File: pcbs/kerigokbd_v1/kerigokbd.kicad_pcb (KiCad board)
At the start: 2 copper layers, 139.5 x 92 mm, 83 parts, among them J1 USB4520-03-0-A, J2 Conn_01x04, J3 Conn_01x03, J4 SJ-3501-SMT-TR, SW1 SW_Push, SW10 SW_Push, SW11 SW_Push, SW12 SW_Push, SW13 SW_Push, SW14 SW_Push, SW15 SW_Push, SW16 SW_Push, SW17 SW_Push, SW18 SW_Push, SW19 SW_Push, SW2 SW_Push, SW20 SW_Push, SW21 SW_Push, SW22 SW_Push, SW23 SW_Push, SW24 SW_Push, SW3 SW_Push, SW4 SW_Push, SW5 SW_Push, SW6 SW_Push, SW7 SW_Push, SW8 SW_Push, SW9 SW_Push, U1 TLV75533PDBVR, U2 RP2040, U3 W25Q16JVUXIQ, Y1 12MHz

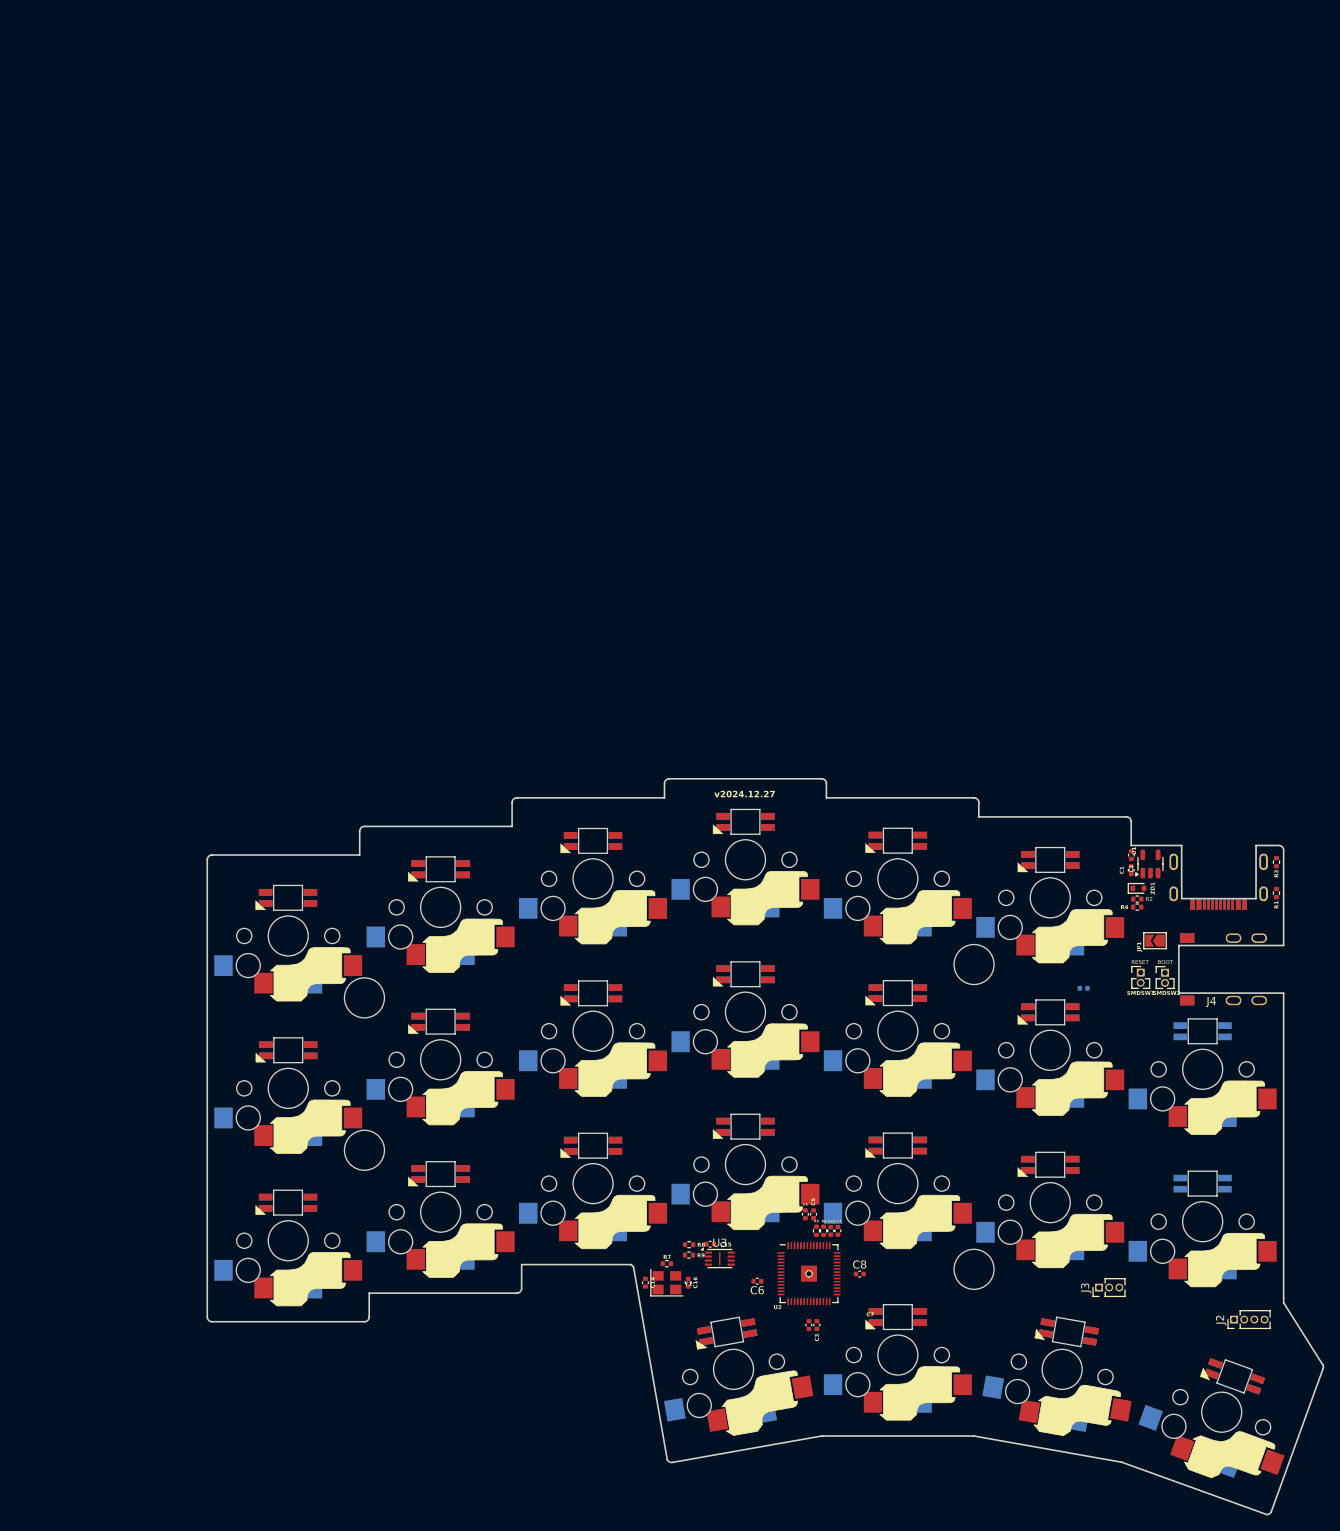
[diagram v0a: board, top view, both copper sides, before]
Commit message: update pcb
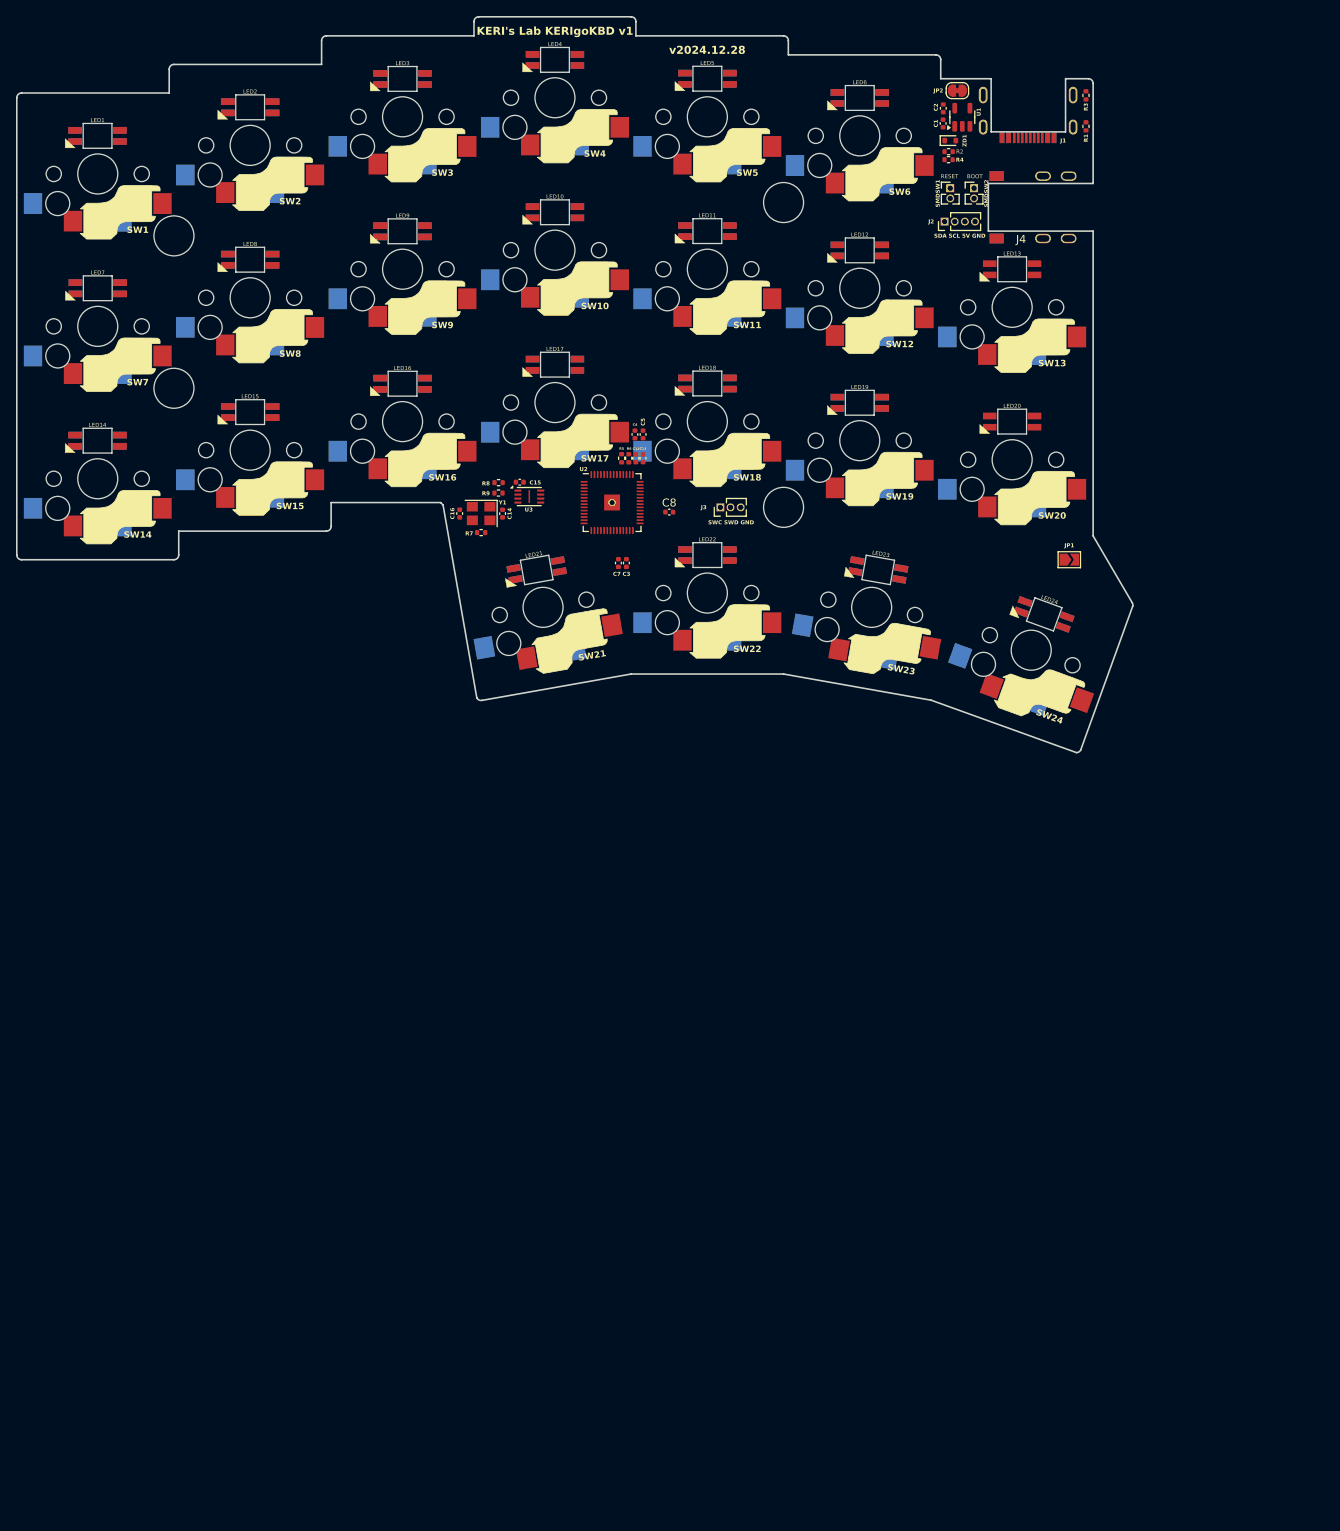
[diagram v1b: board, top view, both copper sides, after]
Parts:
- removed C11, C6: 100n, Capacitor_SMD:C_0402_1005Metric
- added JP2: LED_EN, Jumper:SolderJumper-2_P1.3mm_Bridged_RoundedPad1.0x1.5mm, F.Cu at (133.3, 24.4)
- J1, LED1, LED10, LED11, LED12, LED13, LED14, LED15, LED16, LED17, LED18, LED19, LED2, LED20, LED21, LED22, LED23, LED24, LED3, LED4, LED5, LED6, LED7, LED8, LED9, SW1, SW10, SW11, SW12, SW13, SW14, SW15, SW16, SW17, SW18, SW19, SW2, SW20, SW21, SW22, SW23, SW24, SW3, SW4, SW5, SW6, SW7, SW8, SW9: moved to F.Cu
- J2: value Conn_01x04 -> SDA SCL 5V GND
- J3: value Conn_01x03 -> SWC SWD GND
- moved J2 141.9 mm to (131.7, 40.7)
- moved J3 108.4 mm to (103.7, 76.5)
- moved SMDSW2 100.9 mm to (135.4, 36.6)
- moved SMDSW1 100.9 mm to (132.4, 36.6)
- moved C16 100.3 mm to (71.1, 77.2), turned to 90 degrees
- moved C4 99.8 mm to (93.0, 67.3)
- moved C5 99.8 mm to (94.0, 67.3)
- moved C12 99.6 mm to (93.1, 70.3)
- moved C13 99.6 mm to (94.0, 70.3)
- moved R5 99.6 mm to (91.3, 70.3)
- moved R6 99.6 mm to (92.2, 70.3)
- moved U2 99.5 mm to (90.2, 75.9)
- moved Y1 98.9 mm to (73.8, 77.2), turned to 180 degrees
- moved J1 98.8 mm to (142.2, 24.9), turned to 180 degrees
- moved R1 98.8 mm to (149.4, 28.8)
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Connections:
- LED1 pad 3: GND -> /LED_GND
- LED10 pad 3: GND -> /LED_GND
- LED11 pad 3: GND -> /LED_GND
- LED12 pad 3: GND -> /LED_GND
- LED13 pad 3: GND -> /LED_GND
- LED14 pad 3: GND -> /LED_GND
- LED15 pad 3: GND -> /LED_GND
- LED16 pad 3: GND -> /LED_GND
- LED17 pad 3: GND -> /LED_GND
- LED18 pad 3: GND -> /LED_GND
- LED19 pad 3: GND -> /LED_GND
- LED2 pad 3: GND -> /LED_GND
- LED20 pad 3: GND -> /LED_GND
- LED21 pad 3: GND -> /LED_GND
- LED22 pad 3: GND -> /LED_GND
- LED23 pad 3: GND -> /LED_GND
- LED24 pad 3: GND -> /LED_GND
- LED3 pad 3: GND -> /LED_GND
- LED4 pad 3: GND -> /LED_GND
- LED5 pad 3: GND -> /LED_GND
- LED6 pad 3: GND -> /LED_GND
- LED7 pad 3: GND -> /LED_GND
- LED8 pad 3: GND -> /LED_GND
- LED9 pad 3: GND -> /LED_GND
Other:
- outline, holes or cut-outs redrawn
- board text added: "KERI's Lab KERIgoKBD v1"
- board text added: "v2024.12.28"
- board text removed: "v2024.12.27"
